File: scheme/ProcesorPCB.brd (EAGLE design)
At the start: 87.3 x 59.7 mm, 28 parts, among them U1 UA78L05ACPKG3, X1 22-23-2031, X12 22-23-2051

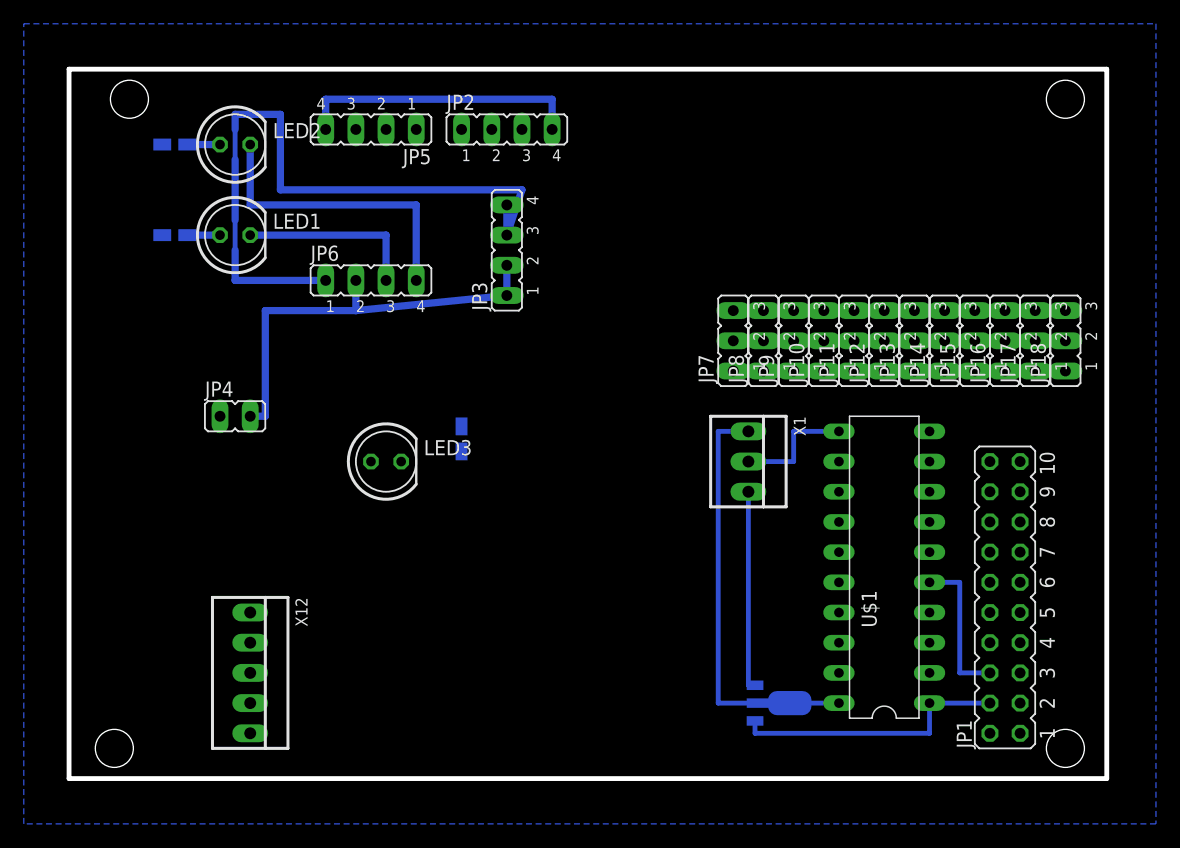
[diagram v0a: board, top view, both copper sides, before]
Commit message: PCB borad almost finished.
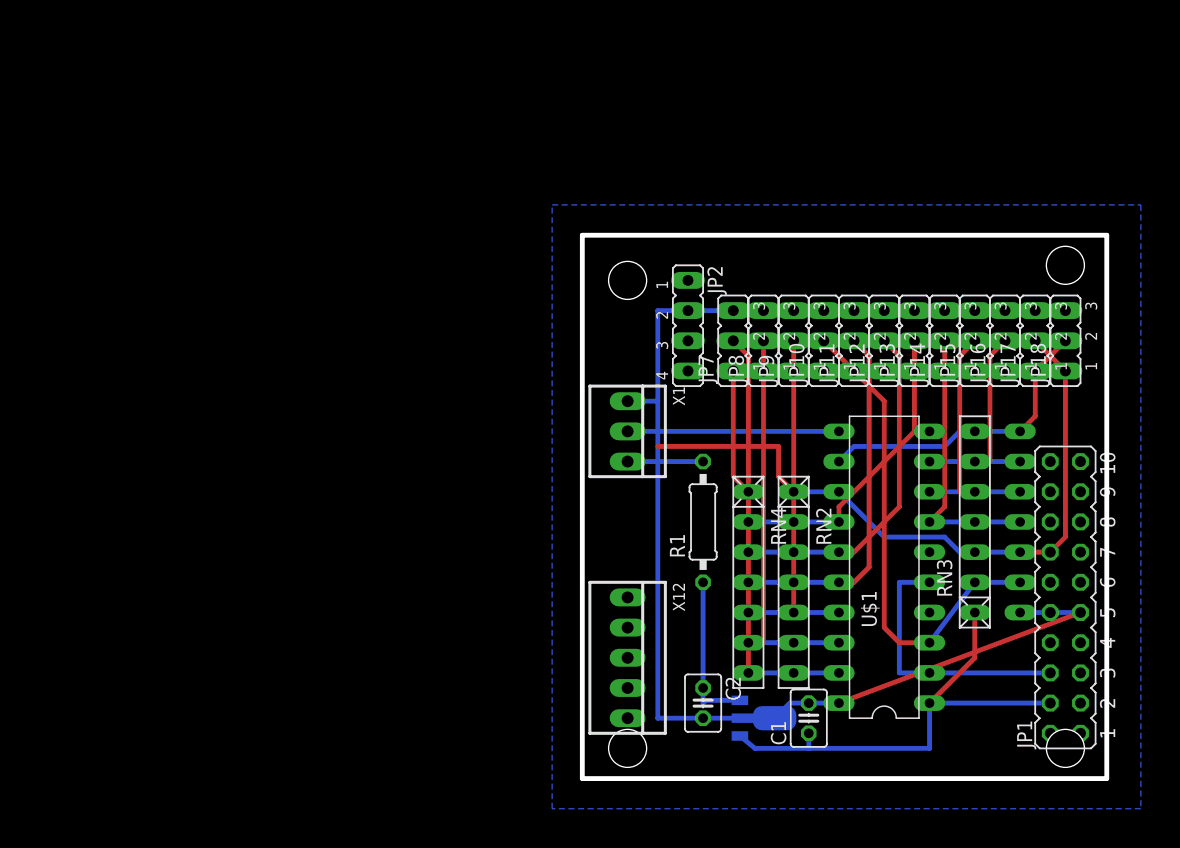
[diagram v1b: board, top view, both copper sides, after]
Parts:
- removed JP3, JP5, JP6: (no value), jumper:JP4
- removed JP4: (no value), jumper:JP1
- removed LED1: Cervena, led:LED5MM
- removed LED2, LED3: Zenena, led:LED5MM
- removed R2, R3: (no value), rcl:R0805W
- added C1: 1uF, resistor:C025-030X050
- added C2: 0.33uF, resistor:C025-030X050
- added RN1, RN2: 15K, resistor-net:RN-7
- added RN3: 22k, resistor-net:RN-7
- added RN4: 22K, resistor-net:RN-7
- R1: device rcl:R0805W -> resistor:0207/10
- moved R1 50.6 mm to (52.1, 21.6), flipped to the top, turned to 90 degrees
- moved X12 31.8 mm to (45.7, 10.2)
- moved JP2 22.5 mm to (50.8, 38.1), turned to 270 degrees
- moved X1 10.5 mm to (45.7, 29.2)
- moved JP1 5.08 mm to (82.5, 15.2)
- moved U1 1.80 mm to (57.1, 5.08)
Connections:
- removed net AN11: JP18.2, U$1.12
- removed net N$3: JP6.4, LED2.K
- removed net N$4: JP6.3, LED1.K
- removed net N$5: LED2.A, R2.2
- removed net N$6: LED1.A, R1.2
- removed net N$8: LED3.K, R3.2
- removed net N$9: JP3.3, JP3.4, JP6.1
- removed net RX: JP2.4, JP5.4
- new net AN11,RX: JP18.2, JP2.4, RN1.7, RN3.7, U$1.12
- net +24V: now also R1.2; no longer U1.3
- net +5V: now also C1.1, RN3.1, RN4.1
- net AN0,PGD: now also RN2.7, RN4.7
- net AN1,PGC: now also RN2.6, RN4.6
- net AN10: now also RN1.3, RN3.3
- net AN2: now also RN2.5, RN4.5
- net AN3: now also RN1.2, RN3.2
- net AN4: now also RN2.4, RN4.4
- net AN5: now also RN2.3, RN4.3
- net AN6: now also RN2.2, RN4.2
- net AN7: now also RN1.4, RN3.4
- net AN8: now also RN1.5, RN3.5
- net AN9: now also RN1.6, RN3.6
- net GND: now also C1.2, C2.2, JP2.2, RN1.1, RN2.1
- net N$2: now also C2.1, R1.1, U1.3; no longer JP3.1, JP3.2, JP4.2, JP6.2
- net TX: no longer JP5.3
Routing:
- net GND: track 63.5 -> 128.2 mm, vias 0 -> 1
- net N$9: track 58.6 -> 0.00 mm
- net AN10: track 0.00 -> 41.8 mm
- net AN3: track 0.00 -> 40.7 mm
- net AN0,PGD: track 0.00 -> 36.1 mm
- net AN1,PGC: track 0.00 -> 34.3 mm
- net AN2: track 0.00 -> 30.5 mm
- net AN4: track 0.00 -> 30.3 mm
- net AN5: track 0.00 -> 28.8 mm
- net +5V: track 51.3 -> 79.4 mm
- net AN11,RX: track 0.00 -> 25.5 mm
- net AN6: track 0.00 -> 25.5 mm
- net N$3: track 25.4 -> 0.00 mm
- net RX: track 24.1 -> 0.00 mm
- net AN7: track 0.00 -> 23.4 mm
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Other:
- board size 87.3 x 59.7 mm -> 44.1 x 45.7 mm
